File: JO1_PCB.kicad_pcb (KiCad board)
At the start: 2 copper layers, 66.5 x 79.5 mm, 25 parts, among them J1 CN8, J10 ESC_PWM, J11 CAN_WCMCU-1051_BLUEPILL, J12 TFT, J13 LM2596_3.3V, J14 LM2596_5V, J2 CN7, J3 CN9, J4 CN10, J5 MPU-6050, J6 CAN_WCMCU-1051_NUCLEO, J7 SERVO, J8 DC_MOTOR, J9 ESC_MOTOR, SW1 SW_Nidec_CAS-120A1, U1 NRF24L01, U2 BP

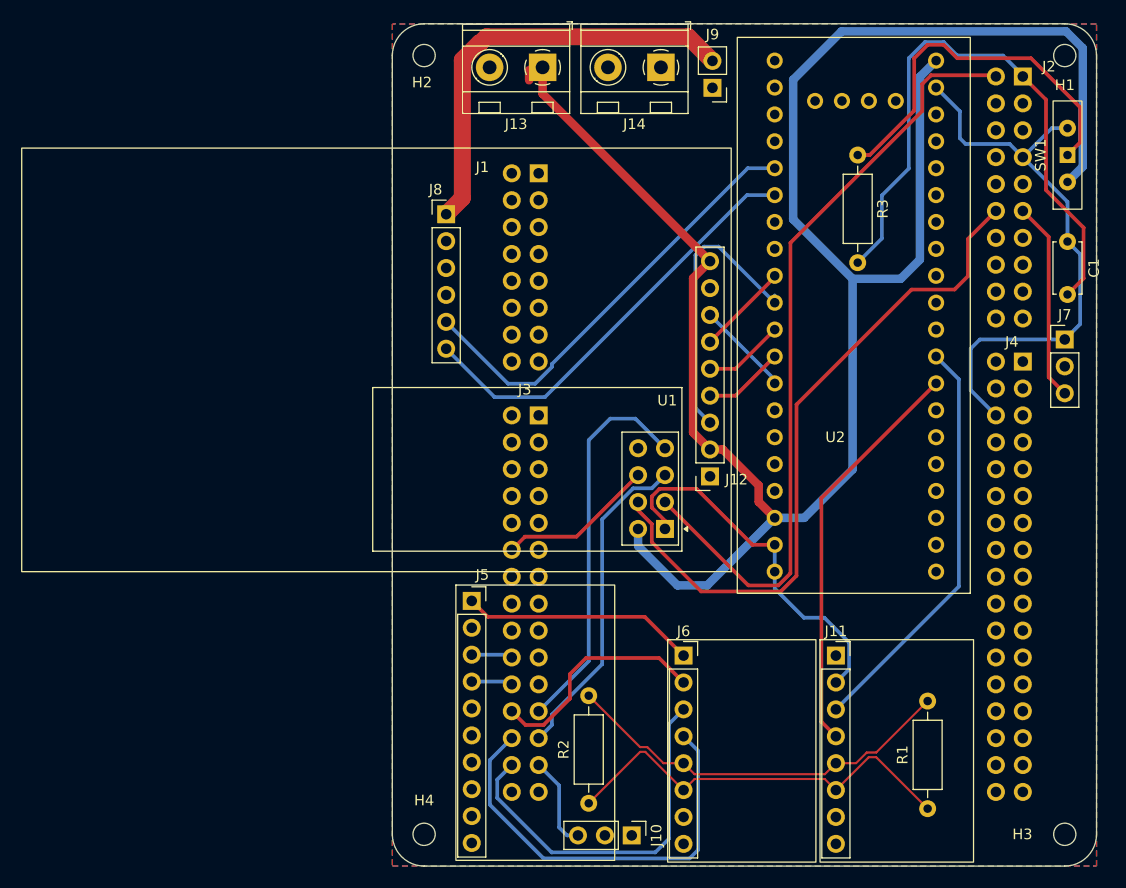
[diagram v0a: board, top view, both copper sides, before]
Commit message: Version Nov 21
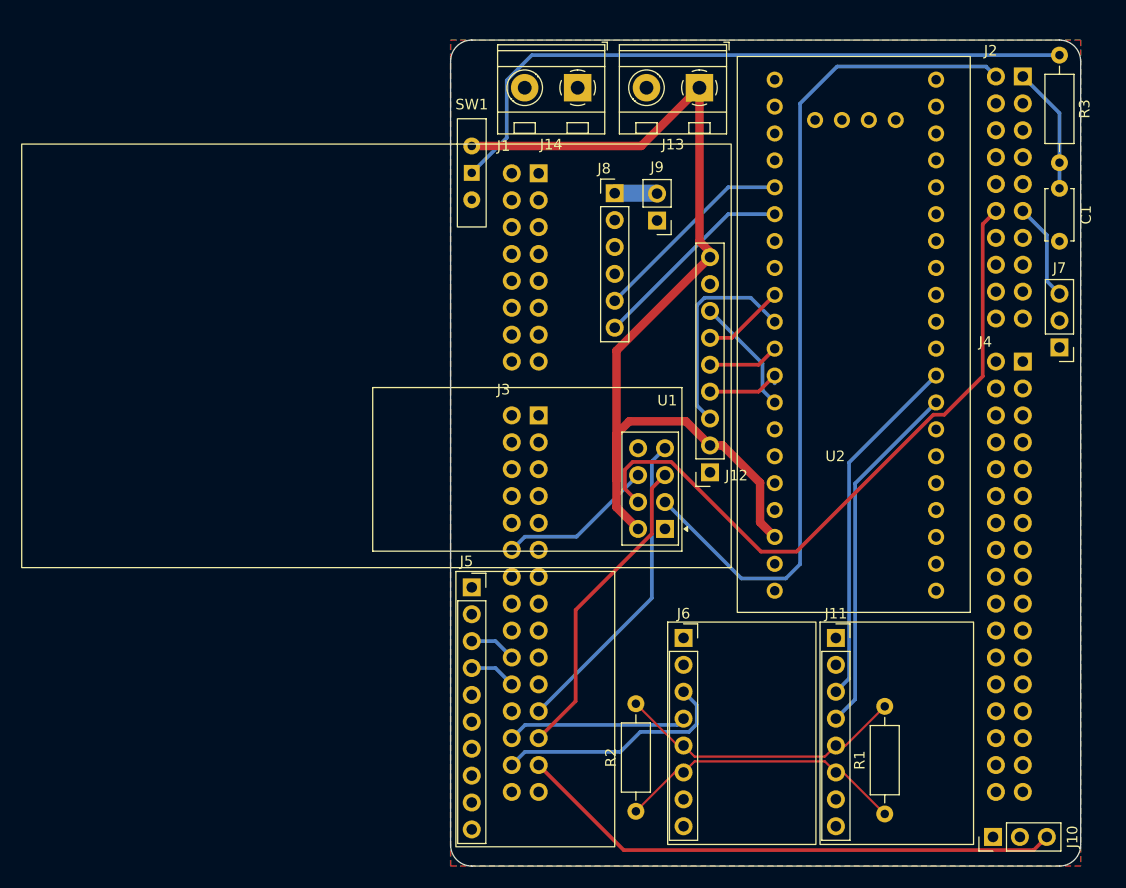
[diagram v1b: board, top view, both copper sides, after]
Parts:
- removed H1, H2, H3, H4: MountingHole, MountingHole:MountingHole_2.1mm
- moved SW1 56.3 mm to (103.0, 72.0), turned to -90 degrees
- moved J10 34.1 mm to (152.2, 134.8), turned to 90 degrees
- moved R3 21.3 mm to (158.5, 60.9)
- moved J8 16.0 mm to (116.5, 74.0)
- moved J13 14.9 mm to (124.5, 64.0)
- moved J9 13.6 mm to (120.5, 76.5)
- moved J14 8.10 mm to (113.0, 64.0)
- moved C1 5.08 mm to (158.5, 73.5)
- moved R2 4.52 mm to (118.5, 132.3)
- moved R1 4.08 mm to (142.0, 132.6)
- moved U2 1.80 mm to (137.3, 90.5)
- moved J11 1.67 mm to (137.4, 116.0)
- moved J6 1.67 mm to (123.0, 116.0)
- moved J5 1.28 mm to (103.0, 111.2)
- moved J7 0.90 mm to (158.5, 88.5), turned to 180 degrees
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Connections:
- C1 pad 1: GND -> Net-(J2-2)
- C1 pad 2: Net-(J2-2) -> GND
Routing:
- net GND: track 111.3 -> 0.00 mm
- net 3.3V: track 191.4 -> 96.8 mm
- net Net-(J2-2): track 57.7 -> 12.1 mm
- net NUCLEO_ESC_TIM14_CH1: track 8.79 -> 51.8 mm
- net MOTOR_VCC: track 40.7 -> 4.02 mm
- net Net-(SW1-B): track 35.7 -> 63.3 mm
- net NUCLEO_FDCAN_RX: track 40.5 -> 17.0 mm
- net BLUEPILL_ENCODER_A: track 42.0 -> 19.6 mm
- net 5V: track 22.1 -> 0.00 mm
- net BLUEPILL_ENCODER_B: track 40.8 -> 19.6 mm
- net NUCLEO_FDCAN_TX: track 35.3 -> 22.6 mm
- net CAN_-: track 39.7 -> 27.5 mm
- net CAN_+: track 37.9 -> 27.5 mm
- net NUCLEO_SERVO_TIM13_CH1: track 18.9 -> 9.24 mm
- net BLUEPILL_TFT_CLK: track 27.1 -> 19.8 mm
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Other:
- board size 66.5 x 79.5 mm -> 59.5 x 78 mm
